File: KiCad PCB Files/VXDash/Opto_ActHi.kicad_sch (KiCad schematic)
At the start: 3 parts, among them U7 DPC817

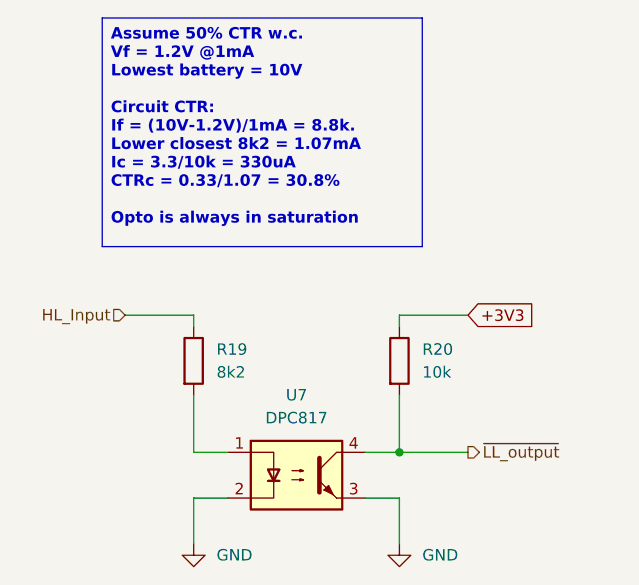
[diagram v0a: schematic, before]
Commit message: ERC corrections, idiot lights
- VXDash : added idiot lights (also to emulator board)
- VXDash : corrected some ERC violations
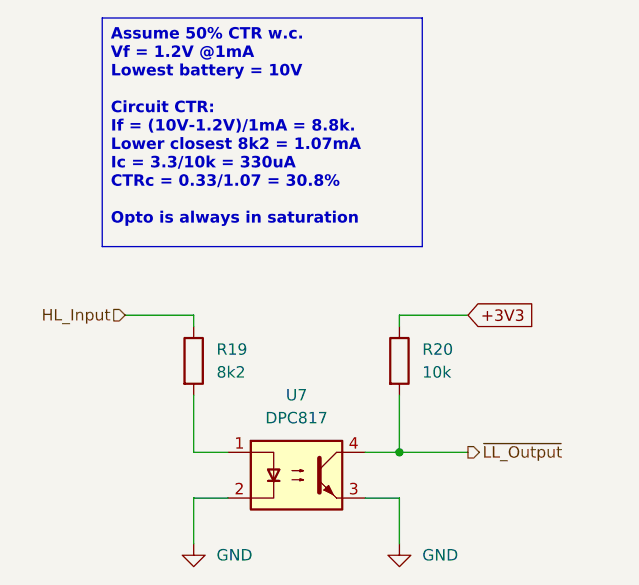
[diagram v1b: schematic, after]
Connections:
- net ~{LL_output} renamed ~{LL_Output}
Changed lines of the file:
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@@
 		)
 	)
-	(hierarchical_label "~{LL_output}"
+	(hierarchical_label "~{LL_Output}"
 		(shape output)
 		(at 157.48 96.52 0)
